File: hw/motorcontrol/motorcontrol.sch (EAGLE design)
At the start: 101 parts, among them J2 USB-MICROB, U1 BTN8982TA, U11 DMG2305UX, U12 BSS138BKS, U2 BTN8982TA, U3 BTN8982TA, U4 CAT24C32WI-GT3, U5 ADG3308, U6 MMDT5401, U7 PTR08060W, U8 IPD90P03P4L-04, U9 ATMEGA32U4

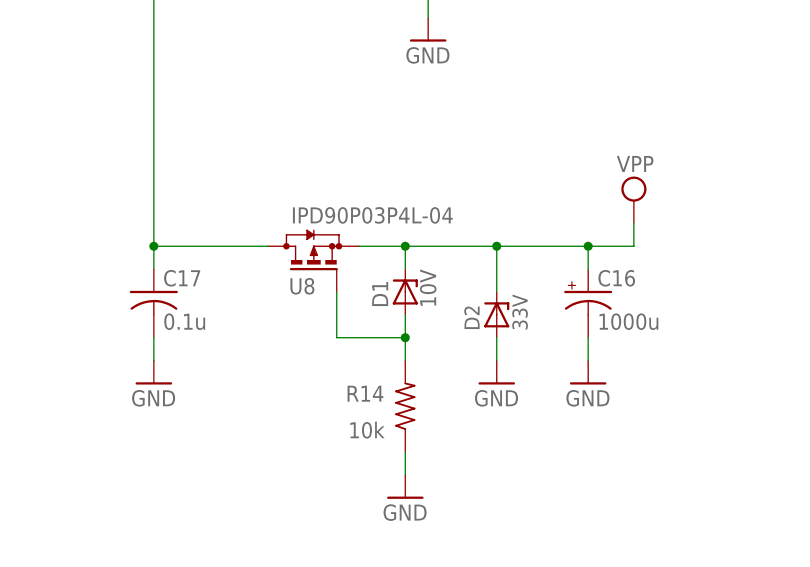
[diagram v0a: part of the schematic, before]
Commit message: backup
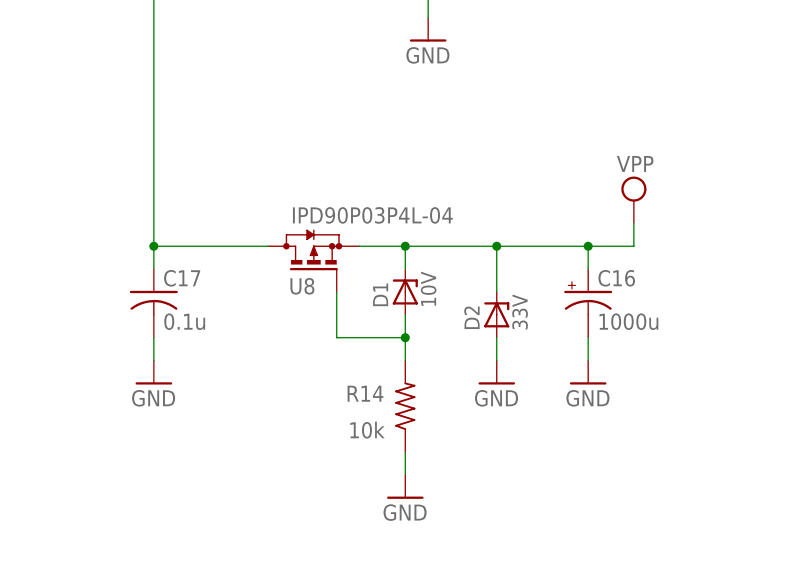
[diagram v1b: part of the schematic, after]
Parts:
- D1: device diode:ZENER-DIODESOD80C -> rpibout:ZENER_DIODESOD123
- D2: device rpibout:SMAZX -> rpibout:ZENER_DIODESMA
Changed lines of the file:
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@@
 <part name="R14" library="resistor" deviceset="R-US_" device="R1206" value="10k"/>
 <part name="GND17" library="supply1" deviceset="GND" device=""/>
-<part name="D1" library="diode" deviceset="ZENER-DIODE" device="SOD80C" value="10V"/>
 <part name="C17" library="resistor" deviceset="C-US" device="C1206" value="0.1u"/>
 <part name="GND18" library="supply1" deviceset="GND" device=""/>
@@
 <part name="U7" library="rpibout" deviceset="PTR08060W" device=""/>
 <part name="C16" library="resistor" deviceset="CPOL-US" device="E5-10.5" value="1000u"/>
-<part name="D2" library="rpibout" deviceset="SMAZX" device="" value="33V"/>
 <part name="R16" library="resistor" deviceset="R-US_" device="R1206" value="10k"/>
 <part name="P+5" library="supply1" deviceset="+5V" device=""/>
@@
 <part name="XTAL1" library="rpibout" deviceset="XTAL" device="ABLS7M2" value="16MHz"/>
 <part name="S1" library="rpibout" deviceset="SWITCH-GND" device=""/>
+<part name="D1" library="rpibout" deviceset="ZENER_DIODE" device="SOD123" value="10V"/>
+<part name="D2" library="rpibout" deviceset="ZENER_DIODE" device="SMA" value="33V"/>
 </parts>
 <sheets>
@@
 </instance>
 <instance part="GND17" gate="1" x="60.96" y="12.7"/>
-<instance part="D1" gate="G$1" x="60.96" y="35.56" rot="R90"/>
 <instance part="C17" gate="G$1" x="33.02" y="35.56"/>
 <instance part="GND18" gate="1" x="33.02" y="25.4"/>
@@
 <instance part="U7" gate="G$1" x="63.5" y="83.82"/>
 <instance part="C16" gate="G$1" x="81.28" y="35.56"/>
-<instance part="D2" gate="G$1" x="71.12" y="33.02" rot="R90"/>
 <instance part="R16" gate="G$1" x="210.82" y="213.36" smashed="yes" rot="R90">
 <attribute name="NAME" x="212.1154" y="216.154" size="1.778" layer="95"/>
@@
 <instance part="XTAL1" gate="G$1" x="129.54" y="175.26" rot="R270"/>
 <instance part="S1" gate="G$1" x="121.92" y="218.44" rot="R270"/>
+<instance part="D1" gate="G$1" x="60.96" y="35.56" rot="R90"/>
+<instance part="D2" gate="G$1" x="71.12" y="33.02" rot="R90"/>
 </instances>
 <busses>
@@
 <wire x1="60.96" y1="27.94" x2="60.96" y2="30.48" width="0.1524" layer="91"/>
 <pinref part="R14" gate="G$1" pin="2"/>
-<pinref part="D1" gate="G$1" pin="A"/>
 <wire x1="60.96" y1="30.48" x2="53.34" y2="30.48" width="0.1524" layer="91"/>
 <wire x1="53.34" y1="30.48" x2="53.34" y2="35.56" width="0.1524" layer="91"/>
@@
 <junction x="60.96" y="30.48"/>
 <pinref part="U8" gate="G$1" pin="G"/>
+<pinref part="D1" gate="G$1" pin="A"/>
 </segment>
 </net>
@@
 <net name="VPP" class="0">
 <segment>
-<pinref part="D1" gate="G$1" pin="C"/>
 <wire x1="55.88" y1="40.64" x2="60.96" y2="40.64" width="0.1524" layer="91"/>
 <wire x1="60.96" y1="40.64" x2="71.12" y2="40.64" width="0.1524" layer="91"/>
@@
 <pinref part="U8" gate="G$1" pin="S"/>
 <pinref part="C16" gate="G$1" pin="+"/>
+<pinref part="D1" gate="G$1" pin="C"/>
 <pinref part="D2" gate="G$1" pin="C"/>
 </segment>
